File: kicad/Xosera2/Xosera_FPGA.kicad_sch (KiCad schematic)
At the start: 95 parts, among them J1 47589-0001, U1 93LC56BT-I/OT, U2 ICE40UP5K-SG48ITR, U3 FT232H, U4 SG-210STF 12.0000ML3, U5 W25Q32JVSSIM, U6 AP2127K-3.3, U7 AP2127K-1.2, U8 SN74AUP2G125DCUR

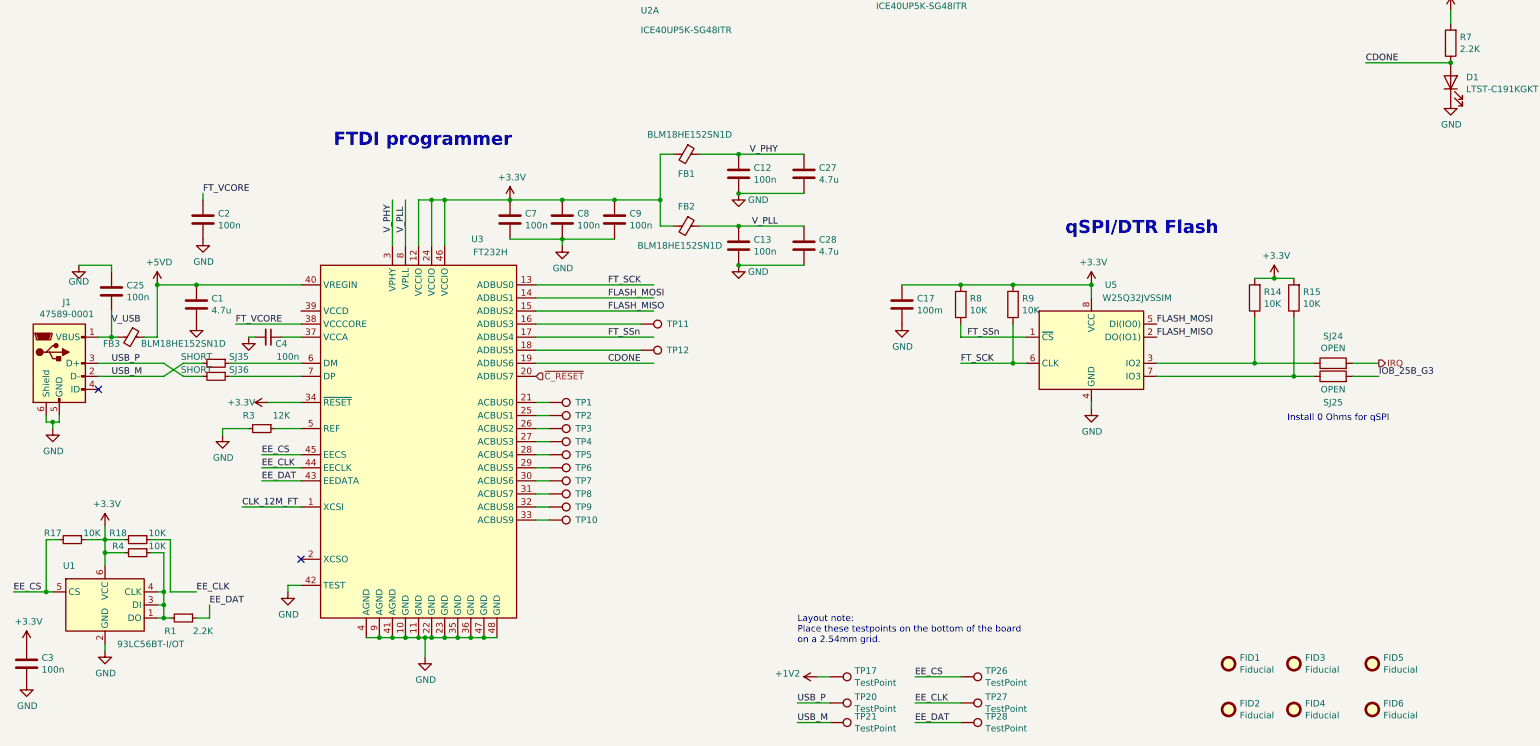
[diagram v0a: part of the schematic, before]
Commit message: Fix Kicad weirdness
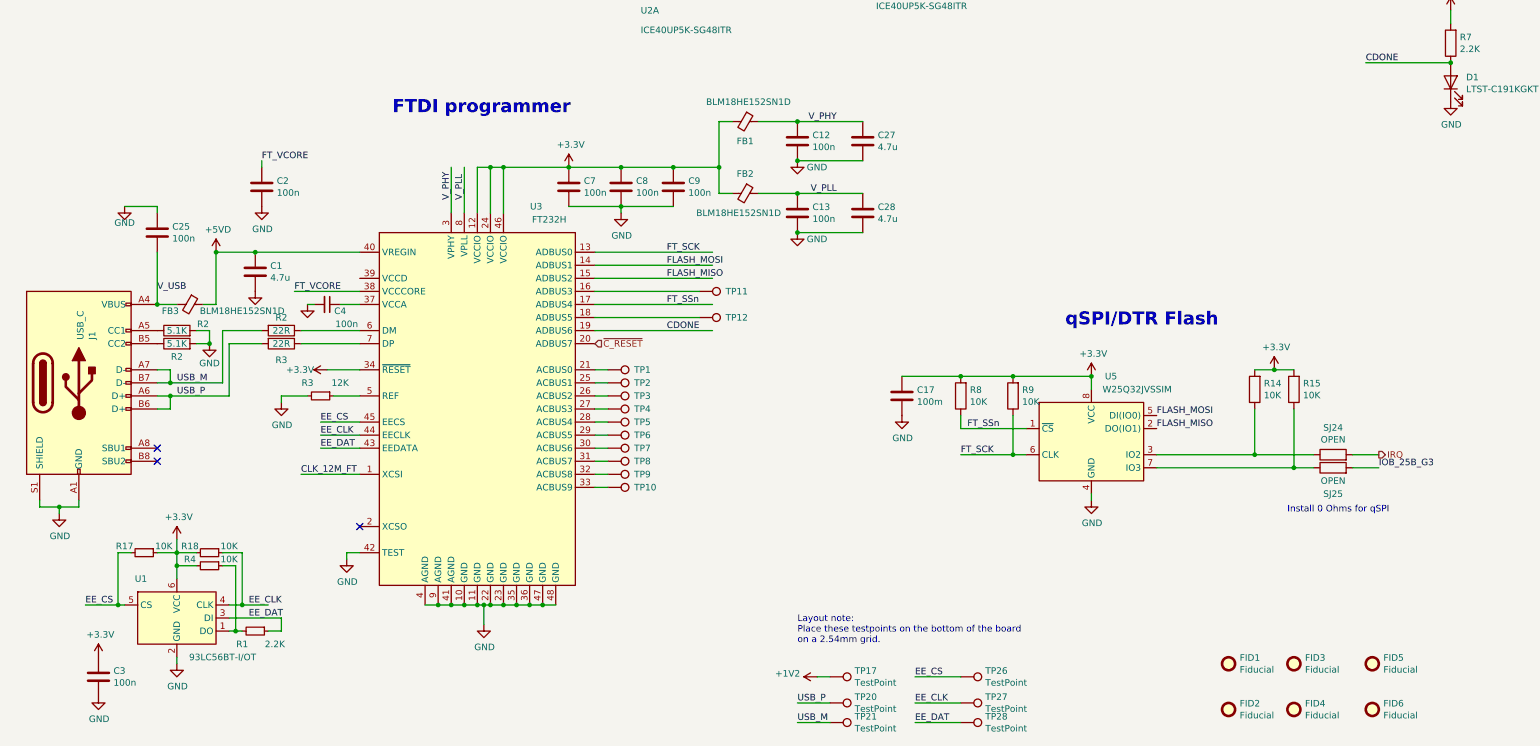
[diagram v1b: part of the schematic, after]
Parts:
- removed J1: 47589-0001, Connector_USB:USB_Micro-AB_Molex_47590-0001, symbol Connector:USB_B_Micro
- removed SJ35, SJ36: SHORT, Jumper:SolderJumper-2_P1.3mm_Bridged2Bar_RoundedPad1.0x1.5mm, symbol Device:R_Small
- added J1: USB_C, Connector_USB:USB_C_Receptacle_Palconn_UTC16-G, symbol Connector:USB_C_Receptacle_USB2.0
- added R2 (x2): 5.1K, Resistor_SMD:R_0805_2012Metric_Pad1.20x1.40mm_HandSolder, symbol Device:R
- added R2, R3: 22R, Resistor_SMD:R_0805_2012Metric_Pad1.20x1.40mm_HandSolder, symbol Device:R
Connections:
- net EE_CLK: now also U1.4 (CLK)
- net EE_DAT: now also U1.3 (DI)
- net GND: now also J1.A1 (GND), J1.A12 (GND), J1.B1 (GND), J1.B12 (GND), J1.S1 (SHIELD), R2.2, R2.2
- net USB_M: now also J1.A7 (D-), J1.B7 (D-), R2.2
- net USB_P: now also J1.A6 (D+), J1.B6 (D+), R3.2
- net V_USB: now also J1.A4 (VBUS), J1.A9 (VBUS), J1.B4 (VBUS), J1.B9 (VBUS)
- net at U3.6 (DM): now also R2.1
- net at U3.7 (DP): now also R3.1
- net at R1.2, R4.1, U1.1 (DO): no longer U1.3 (DI), U1.4 (CLK)
- new net: J1.A5 (CC1), R2.1
- new net: J1.B5 (CC2), R2.1
- no-connect marks 2 -> 3
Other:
- moved on the sheet: C1, C12, C13, C17, C2, C25, C27, C28, C3, C4, C7, C8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
